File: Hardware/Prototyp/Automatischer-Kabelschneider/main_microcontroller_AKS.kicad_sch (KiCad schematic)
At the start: 1 part, among them U2 ESP32-S3-WROOM-2

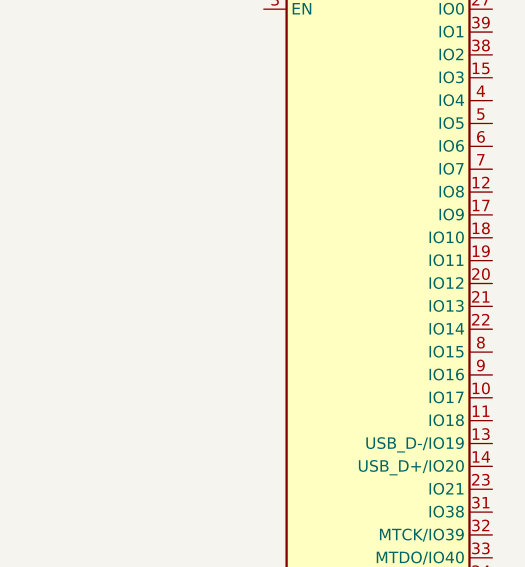
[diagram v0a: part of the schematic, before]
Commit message: 20240410
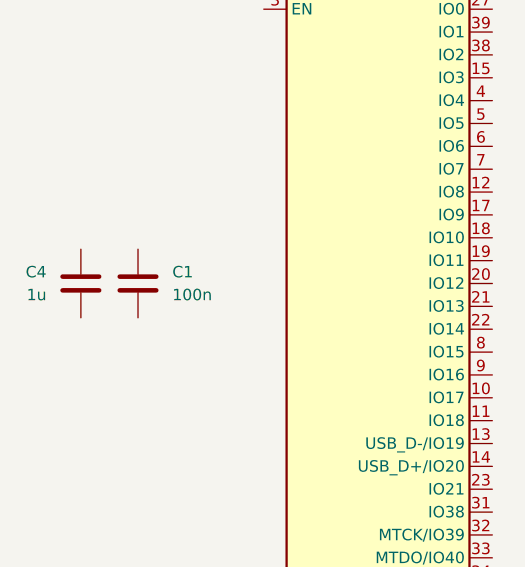
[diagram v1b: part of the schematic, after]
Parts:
- added C1: 100n, Capacitor_SMD:C_0805_2012Metric, symbol Device:C
- added C4: 1u, Capacitor_SMD:C_0805_2012Metric, symbol Device:C
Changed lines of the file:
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@@
+		)
+	)
+	(symbol
+		(lib_id "Device:C")
+		(at 113.03 74.93 0)
+		(unit 1)
+		(exclude_from_sim no)
+		(in_bom yes)
+		(on_board yes)
+		(dnp no)
+		(fields_autoplaced yes)
+		(property "Reference" "C1"
+			(at 116.84 73.6599 0)
+			(effects
+				(font
+					(size 1.27 1.27)
+				)
+				(justify left)
+			)
+		)
+		(property "Value" "100n"
+			(at 116.84 76.1999 0)
+			(effects
+				(font
+					(size 1.27 1.27)
+				)
+				(justify left)
+			)
+		)
+		(property "Footprint" "Capacitor_SMD:C_0805_2012Metric"
+			(at 113.9952 78.74 0)
+			(effects
+				(font
+					(size 1.27 1.27)
+				)
+				(hide yes)
+			)
+		)
+		(property "Datasheet" "~"
+			(at 113.03 74.93 0)
+			(effects
+				(font
+					(size 1.27 1.27)
+				)
+				(hide yes)
+			)
+		)
+		(property "Description" "Unpolarized capacitor"
+			(at 113.03 74.93 0)
+			(effects
+				(font
+					(size 1.27 1.27)
+				)
+				(hide yes)
+			)
+		)
+		(pin "1"
+		)
+		(pin "2"
+		)
+		(instances
+			(project "Automatischer-Kabelschneider"
+				(path "/ff414881-00bc-48a3-bd83-dba8c1da722a/352ad1d3-9b58-40da-b881-d99a3f860b8b"
+					(reference "C1")
+					(unit 1)
+				)
+			)
+		)
+	)
+	(symbol
+		(lib_id "Device:C")
+		(at 106.68 74.93 0)
+		(mirror y)
+		(unit 1)
+		(exclude_from_sim no)
+		(in_bom yes)
+		(on_board yes)
+		(dnp no)
+		(property "Reference" "C4"
+			(at 102.87 73.6599 0)
+			(effects
+				(font
+					(size 1.27 1.27)
+				)
+				(justify left)
+			)
+		)
+		(property "Value" "1u"
+			(at 102.87 76.1999 0)
+			(effects
+				(font
+					(size 1.27 1.27)
+				)
+				(justify left)
+			)
+		)
+		(property "Footprint" "Capacitor_SMD:C_0805_2012Metric"
+			(at 105.7148 78.74 0)
+			(effects
+				(font
+					(size 1.27 1.27)
+				)
+				(hide yes)
+			)
+		)
+		(property "Datasheet" "~"
+			(at 106.68 74.93 0)
+			(effects
+				(font
+					(size 1.27 1.27)
+				)
+				(hide yes)
+			)
+		)
+		(property "Description" "Unpolarized capacitor"
+			(at 106.68 74.93 0)
+			(effects
+				(font
+					(size 1.27 1.27)
+				)
+				(hide yes)
+			)
+		)
+		(pin "1"
+		)
+		(pin "2"
+		)
+		(instances
+			(project "Automatischer-Kabelschneider"
+				(path "/ff414881-00bc-48a3-bd83-dba8c1da722a/352ad1d3-9b58-40da-b881-d99a3f860b8b"
+					(reference "C4")
+					(unit 1)
+				)
+			)
 		)
 	)

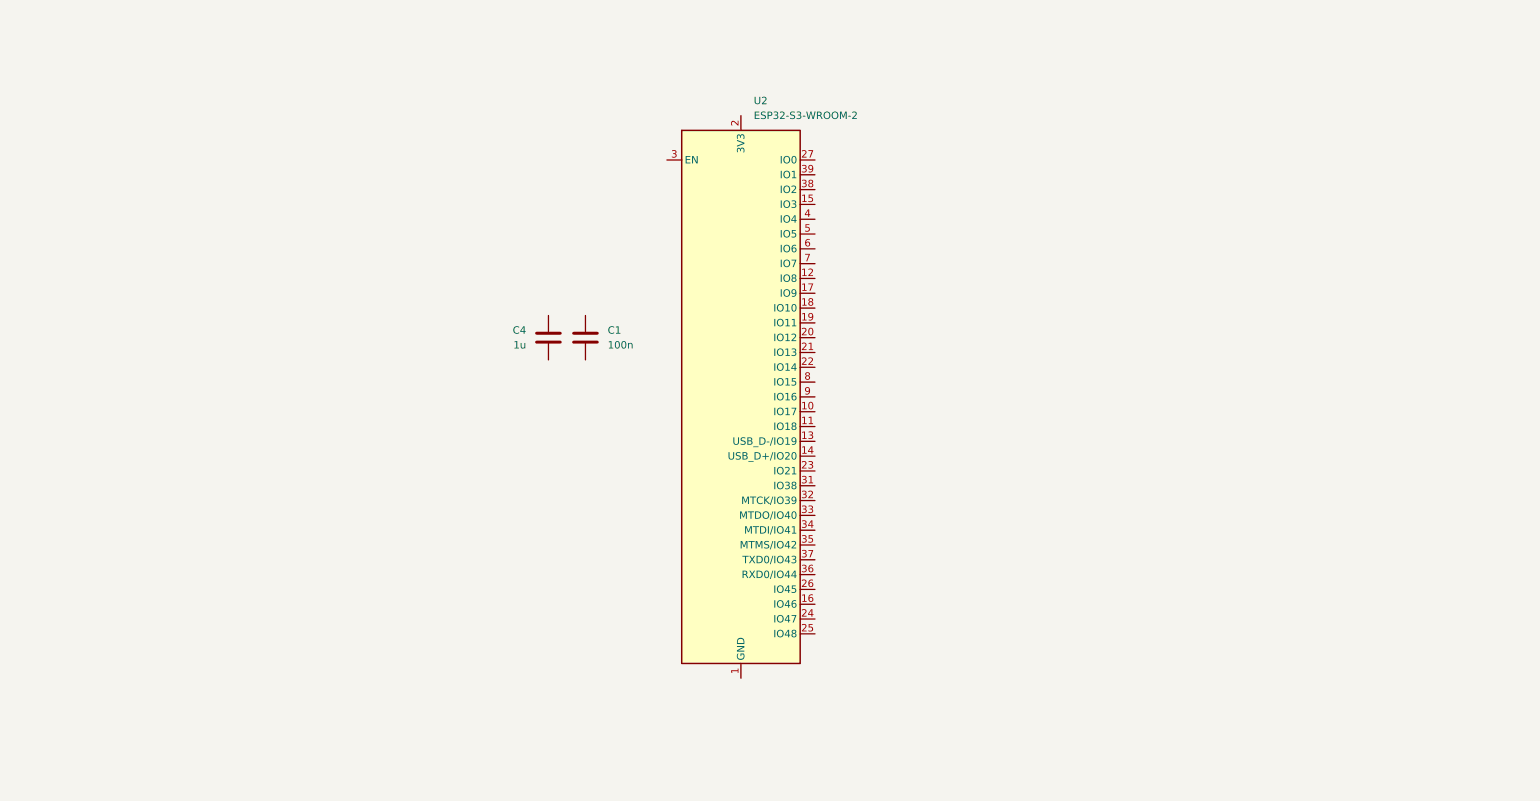
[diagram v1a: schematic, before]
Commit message: 20240415
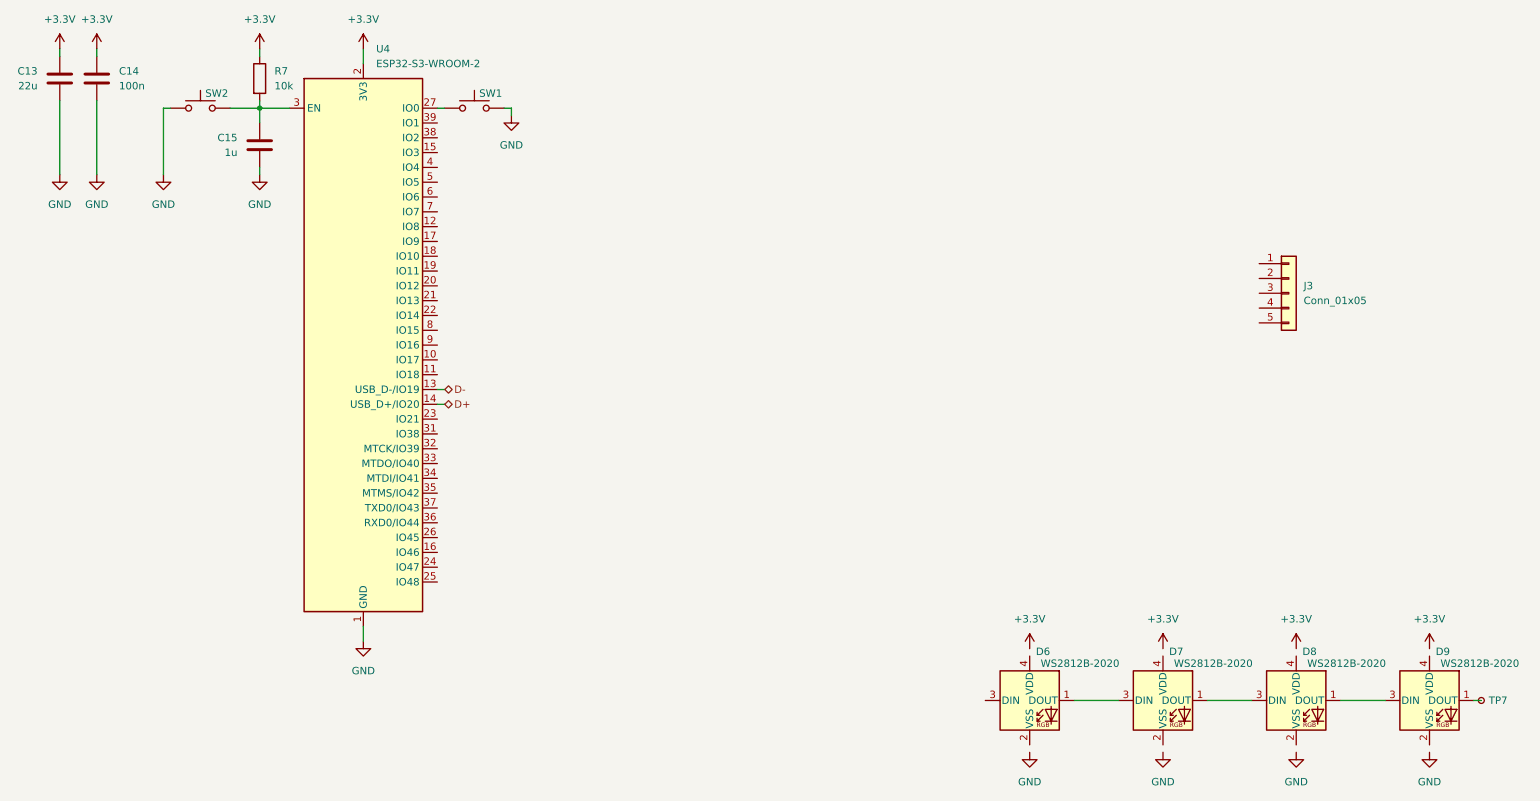
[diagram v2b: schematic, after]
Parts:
- added C15: 1u, Capacitor_SMD:C_0805_2012Metric, symbol Device:C
- added D6, D7, D8, D9: WS2812B-2020, LED_SMD:LED_WS2812B-2020_PLCC4_2.0x2.0mm, symbol LED:WS2812B-2020
- added J3: Conn_01x05, Connector_PinHeader_2.54mm:PinHeader_1x05_P2.54mm_Vertical, symbol Connector_Generic:Conn_01x05
- added R7: 10k, Resistor_SMD:R_0805_2012Metric, symbol Device:R
- added SW1, SW2: SW_Push, Button_Switch_SMD:SW_Push_1P1T_NO_6x6mm_H9.5mm, symbol Switch:SW_Push
- added TP7: TestPoint_Small, TestPoint:TestPoint_Pad_D1.0mm, symbol Connector:TestPoint_Small
- C13: renamed from C4; value 1u -> 22u
- renumbered C1 to C14, U2 to U4
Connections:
- net GND: now reaches U4.1 (GND), U4.40 (GND), U4.41 (GND)
- net GND: now also C13.2, C14.2, C15.2, SW1.2, SW2.1
- net D-: now reaches U4.13 (USB_D-/IO19)
- net D+: now reaches U4.14 (USB_D+/IO20)
- net +3.3V: now reaches U4.2 (3V3)
- net +3.3V: now also C13.1, C14.1, R7.1
- net at U4.27 (IO0): now also SW1.1
- net at U4.3 (EN): now also C15.1, R7.2, SW2.2
- new net: D9.1 (DOUT), TP7.1
- new net: D8.1 (DOUT), D9.3 (DIN)
- new net: D7.1 (DOUT), D8.3 (DIN)
- new net: D6.1 (DOUT), D7.3 (DIN)
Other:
- moved on the sheet: C13, C14, U4
